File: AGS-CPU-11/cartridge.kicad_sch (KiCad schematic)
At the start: 14 parts, among them P1 GameBoyAdvance_Cartridge_Moun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, SW13 GameBoy_SW_DPST

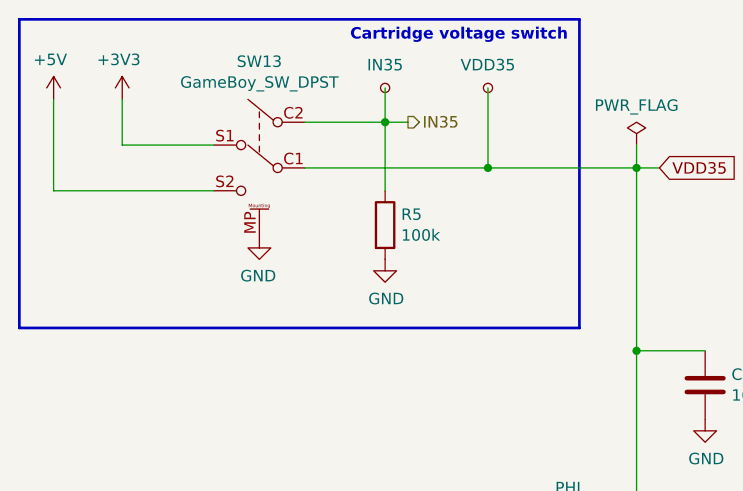
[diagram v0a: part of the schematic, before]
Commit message: Update to latest KiCad
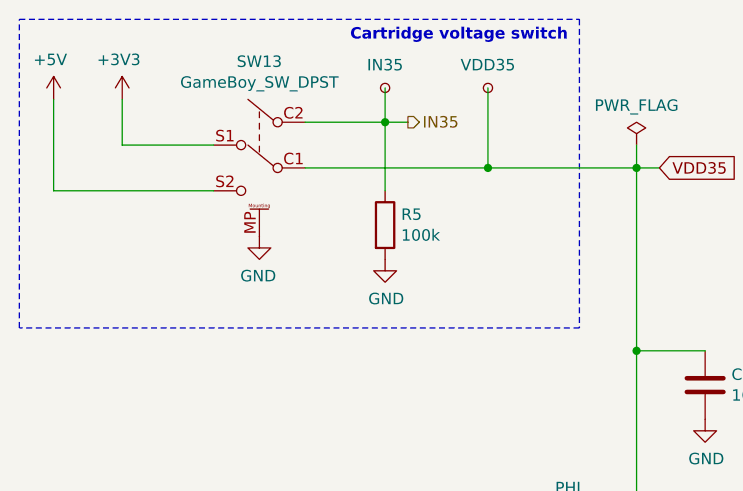
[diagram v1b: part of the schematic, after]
